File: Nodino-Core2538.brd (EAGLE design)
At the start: 27.9 x 25.4 mm, 21 parts, among them CON1 NODINO-JTAGMODULE, CON2 USB-OTG_SHIELD, IC1 CC2538, IC2 AP733333SAG, Q1 32MHz, Q2 32.768kHz

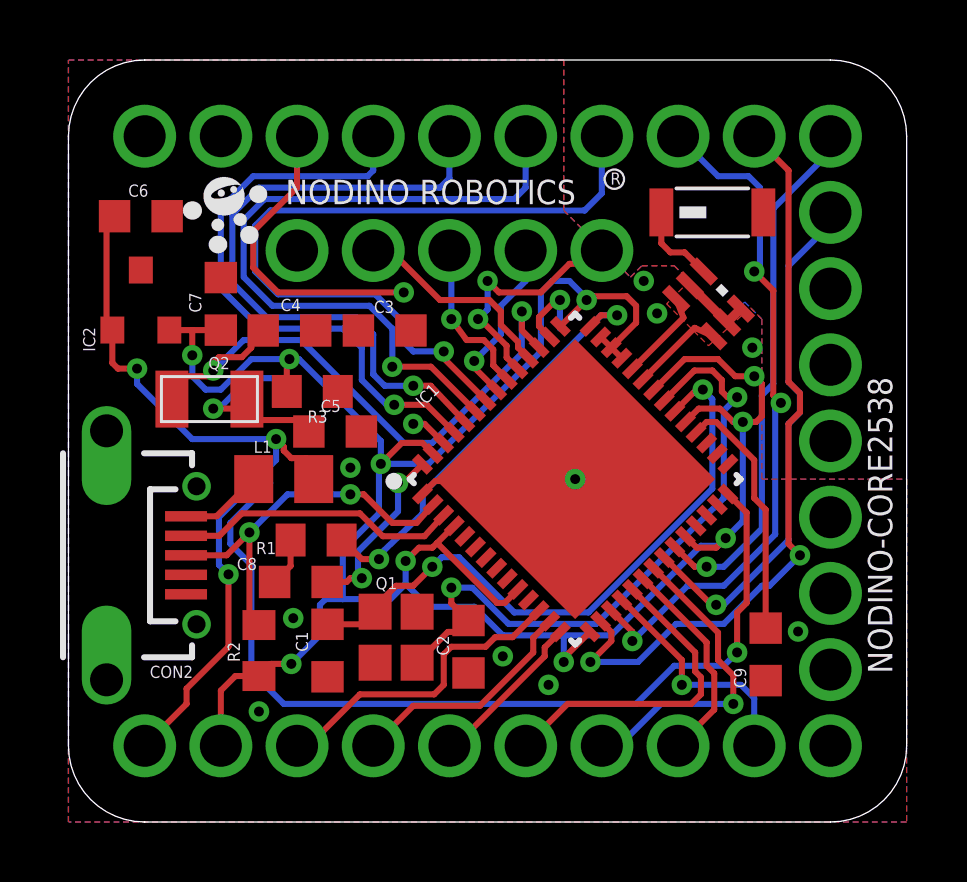
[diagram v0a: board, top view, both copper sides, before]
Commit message: update for D2-D6
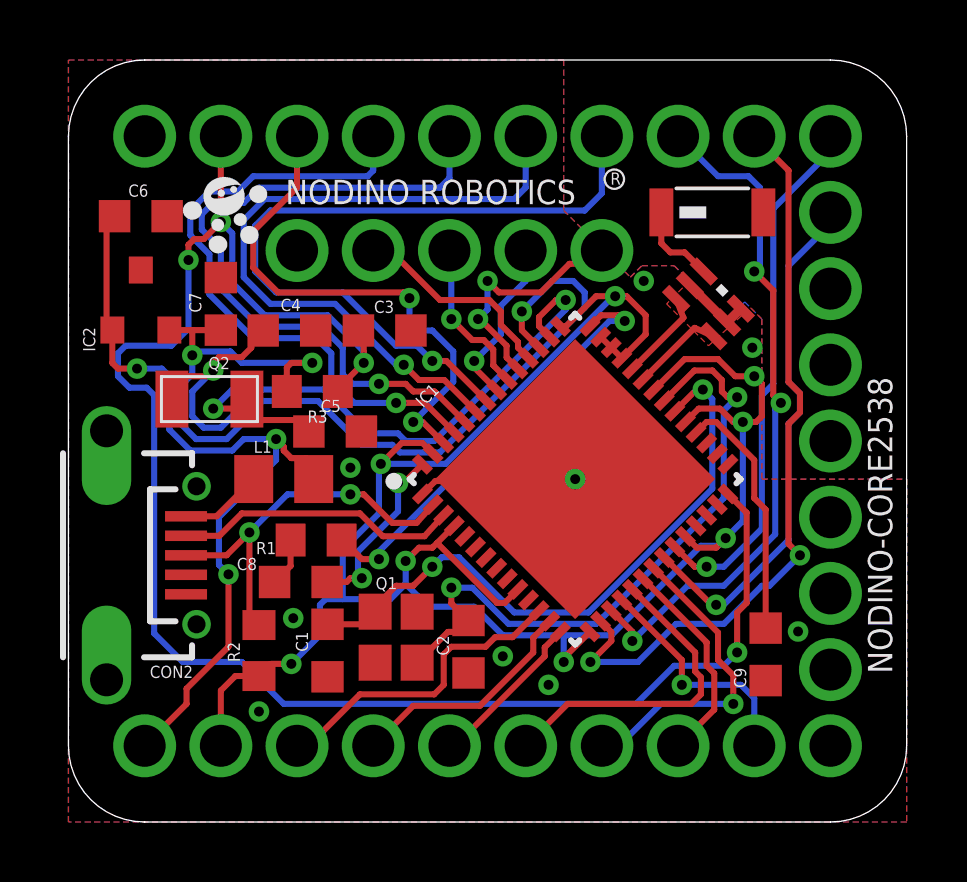
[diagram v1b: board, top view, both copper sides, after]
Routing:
- net NRST: track 30.2 -> 57.1 mm, vias 1 -> 4
- net 32K1: track 10.6 -> 21.4 mm
- net 32K2: track 20.9 -> 27.5 mm
- net PB1: track 11.6 -> 17.5 mm
- net PB2: track 19.8 -> 21.4 mm
- net PB3: track 21.9 -> 23.4 mm
- net +5V: track 26.3 -> 27.4 mm
- net PB4: track 23.8 -> 23.0 mm
- net PB5: track 25.4 -> 24.9 mm
- net GND: vias 10 -> 9

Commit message: final version, but still missing A0-A5 and AREF
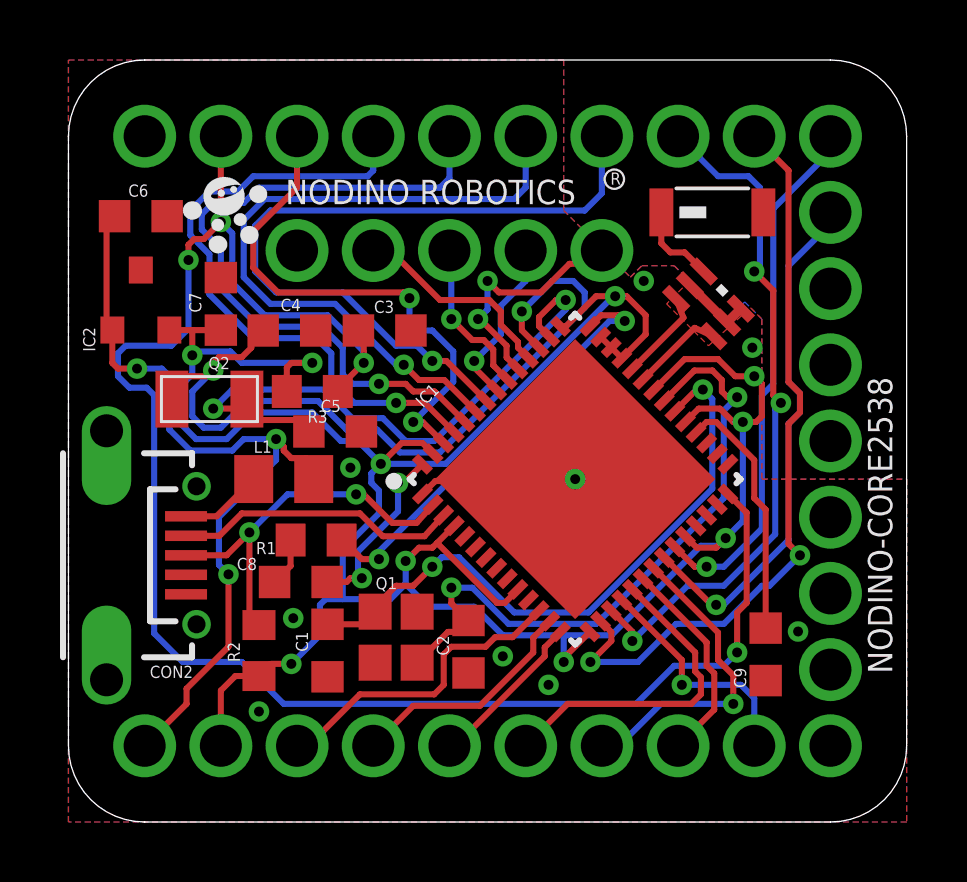
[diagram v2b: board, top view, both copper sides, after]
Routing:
- net +3V3: track 83.3 -> 88.6 mm
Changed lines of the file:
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@@
 <via x="8.128" y="15.3035" extent="1-16" drill="0.3302"/>
 <wire x1="9.144" y1="9.0805" x2="10.3505" y2="10.287" width="0.2032" layer="16"/>
-<wire x1="10.3505" y1="10.287" x2="10.3505" y2="11.8745" width="0.2032" layer="16"/>
 <via x="10.414" y="11.938" extent="1-16" drill="0.3302"/>
 <wire x1="12.153384375" y1="12.278528125" x2="11.7954125" y2="12.6365" width="0.2032" layer="1"/>
 <wire x1="11.7954125" y1="12.6365" x2="11.1125" y2="12.6365" width="0.2032" layer="1"/>
 <wire x1="11.1125" y1="12.6365" x2="10.414" y2="11.938" width="0.2032" layer="1"/>
-<wire x1="10.3505" y1="11.8745" x2="10.414" y2="11.938" width="0.2032" layer="16"/>
 <wire x1="5.7785" y1="15.3035" x2="8.128" y2="15.3035" width="0.2032" layer="16"/>
 <wire x1="18.161" y1="17.526" x2="12.573" y2="11.938" width="0.2032" layer="16"/>
@@
 <wire x1="16.58466875" y1="16.52116875" x2="17.5895" y2="17.526" width="0.2032" layer="1"/>
 <wire x1="17.5895" y1="17.526" x2="18.2245" y2="17.526" width="0.2032" layer="1"/>
-<wire x1="6.096" y1="13.589" x2="5.2705" y2="12.7635" width="0.2032" layer="16"/>
+<wire x1="6.1595" y1="13.6525" x2="5.2705" y2="12.7635" width="0.2032" layer="16"/>
 <wire x1="5.2705" y1="12.7635" x2="4.2545" y2="12.7635" width="0.2032" layer="16"/>
 <wire x1="4.2545" y1="12.7635" x2="3.7465" y2="13.2715" width="0.2032" layer="16"/>
@@
 <wire x1="7.278" y1="15.152" x2="7.4295" y2="15.3035" width="0.2032" layer="1"/>
 <wire x1="7.4295" y1="15.3035" x2="8.128" y2="15.3035" width="0.2032" layer="1"/>
-<wire x1="10.414" y1="11.938" x2="7.278" y2="14.351" width="0" layer="19" extent="1-1"/>
+<wire x1="10.3505" y1="10.287" x2="10.3505" y2="11.049" width="0.2032" layer="16"/>
+<wire x1="10.3505" y1="11.049" x2="10.0965" y2="11.303" width="0.2032" layer="16"/>
+<wire x1="10.414" y1="11.938" x2="10.0965" y2="11.6205" width="0.2032" layer="16"/>
+<wire x1="10.0965" y1="11.6205" x2="10.0965" y2="11.303" width="0.2032" layer="16"/>
+<wire x1="10.414" y1="11.938" x2="9.652" y2="12.7" width="0.2032" layer="16"/>
+<wire x1="9.652" y1="12.7" x2="9.0805" y2="12.7" width="0.2032" layer="16"/>
+<wire x1="9.0805" y1="12.7" x2="8.128" y2="13.6525" width="0.2032" layer="16"/>
+<wire x1="8.128" y1="13.6525" x2="6.1595" y2="13.6525" width="0.2032" layer="16"/>
 </signal>
 <signal name="CS2">
@@
 <contactref element="IC1" pad="2"/>
 <via x="6.0325" y="9.652" extent="1-16" drill="0.3302"/>
-<via x="9.398" y="10.922" extent="1-16" drill="0.3302"/>
+<via x="9.5885" y="10.922" extent="1-16" drill="0.3302"/>
 <wire x1="11.604915625" y1="9.9695" x2="12.153384375" y2="10.58146875" width="0.2032" layer="1"/>
 <wire x1="11.604915625" y1="9.9695" x2="10.795" y2="9.9695" width="0.2032" layer="1"/>
@@
 <wire x1="5.2705" y1="8.89" x2="6.0325" y2="9.652" width="0.2032" layer="1"/>
 <wire x1="6.0325" y1="9.652" x2="7.3025" y2="10.922" width="0.2032" layer="16"/>
-<wire x1="7.3025" y1="10.922" x2="9.398" y2="10.922" width="0.2032" layer="16"/>
-<wire x1="9.398" y1="10.922" x2="9.8425" y2="10.922" width="0.2032" layer="1"/>
+<wire x1="7.3025" y1="10.922" x2="9.5885" y2="10.922" width="0.2032" layer="16"/>
+<wire x1="9.5885" y1="10.922" x2="9.8425" y2="10.922" width="0.2032" layer="1"/>
 <wire x1="9.8425" y1="10.922" x2="10.795" y2="9.9695" width="0.2032" layer="1"/>
 </signal>
@@
 <wire x1="8.509" y1="14.4145" x2="5.461" y2="14.4145" width="0.2032" layer="16"/>
 <wire x1="5.461" y1="14.4145" x2="4.826" y2="13.7795" width="0.2032" layer="16"/>
-<wire x1="8.509" y1="14.4145" x2="9.9695" y2="12.954" width="0.2032" layer="16"/>
-<wire x1="9.9695" y1="12.954" x2="10.9855" y2="12.954" width="0.2032" layer="16"/>
-<wire x1="10.9855" y1="12.954" x2="11.2395" y2="12.7" width="0.2032" layer="16"/>
+<wire x1="8.509" y1="14.4145" x2="9.4615" y2="13.462" width="0.2032" layer="16"/>
+<wire x1="9.4615" y1="13.462" x2="10.4775" y2="13.462" width="0.2032" layer="16"/>
+<wire x1="10.4775" y1="13.462" x2="11.2395" y2="12.7" width="0.2032" layer="16"/>
 <wire x1="11.2395" y1="12.7" x2="12.192" y2="12.7" width="0.2032" layer="16"/>
 </signal>
@@
 <wire x1="8.3185" y1="14.0335" x2="5.969" y2="14.0335" width="0.2032" layer="16"/>
 <wire x1="5.969" y1="14.0335" x2="5.08" y2="13.1445" width="0.2032" layer="16"/>
-<wire x1="8.3185" y1="14.0335" x2="9.779" y2="12.573" width="0.2032" layer="16"/>
-<wire x1="9.779" y1="12.573" x2="10.795" y2="12.573" width="0.2032" layer="16"/>
-<wire x1="10.795" y1="12.573" x2="11.049" y2="12.319" width="0.2032" layer="16"/>
+<wire x1="8.3185" y1="14.0335" x2="9.271" y2="13.081" width="0.2032" layer="16"/>
+<wire x1="9.271" y1="13.081" x2="10.287" y2="13.081" width="0.2032" layer="16"/>
+<wire x1="10.287" y1="13.081" x2="11.049" y2="12.319" width="0.2032" layer="16"/>
 <wire x1="11.049" y1="12.319" x2="12.3825" y2="12.319" width="0.2032" layer="16"/>
 </signal>
